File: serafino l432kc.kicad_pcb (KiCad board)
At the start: 4 copper layers, 17.8 x 35.6 mm, 34 parts, among them J1 USB_B_Micro, J2 Conn_01x14, J3 Conn_01x14, Q1 SI3401A-TP, SW1 SW_Push, SW2 SW_Push, U1 AP2112K-3.3, U2 USBLC6-2SC6, U3 STM32L432KCUx, Y1 32.768K

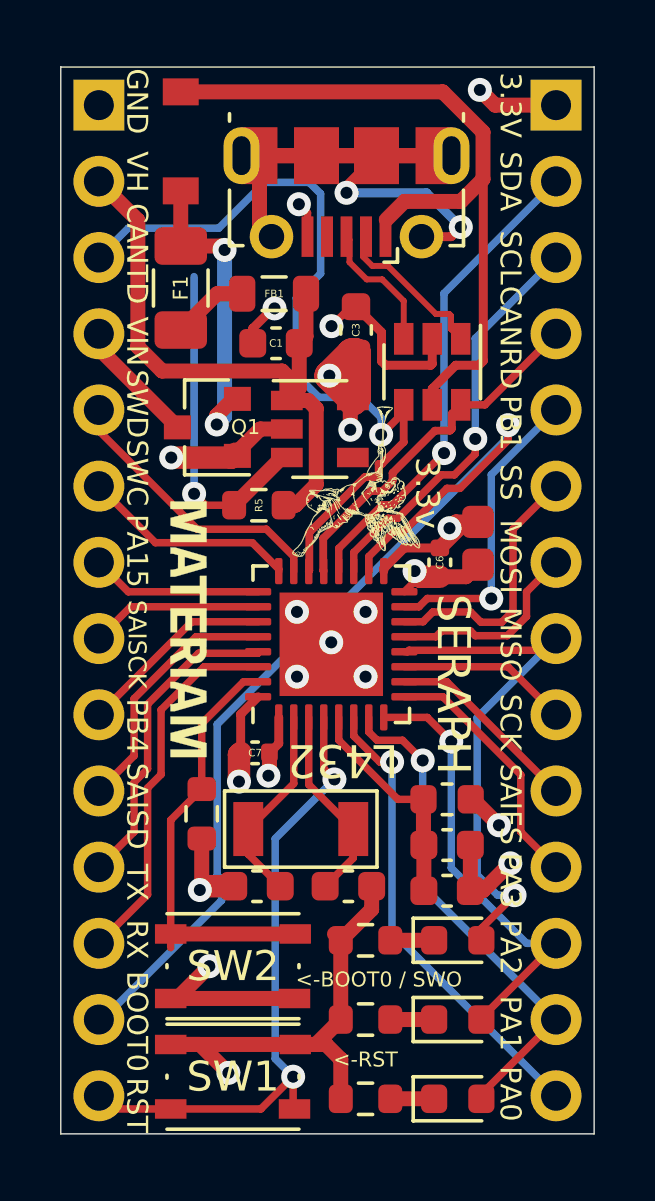
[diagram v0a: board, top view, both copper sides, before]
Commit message: Finished back labels
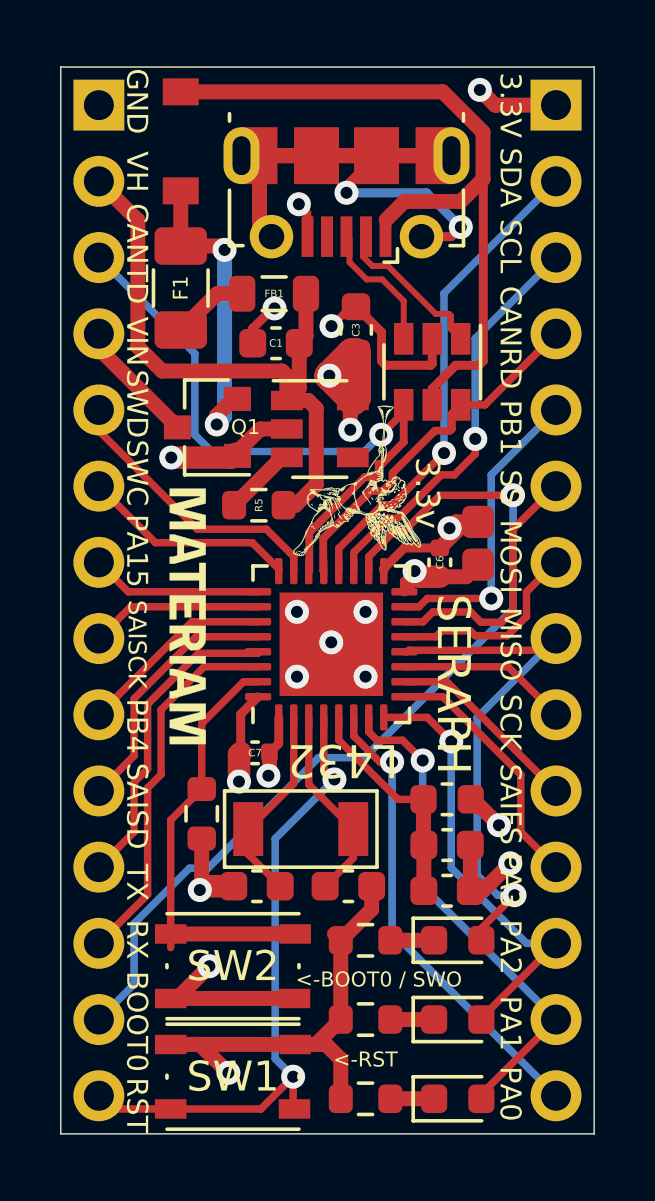
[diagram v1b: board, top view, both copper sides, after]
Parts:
- removed the G*** at (197.5, 98.0)
- moved G*** 0.43 mm to (191.7, 109.4)
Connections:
- net EN renamed Net-(R5-Pad2)
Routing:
- net Net-(R5-Pad2): track 11.1 -> 2.42 mm, vias 1 -> 0
- net CAN_TD: track 27.4 -> 22.4 mm
- net PA8: track 33.0 -> 30.6 mm
- net GND: track 42.2 -> 43.7 mm
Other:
- board text added: "* STM32L432KC ARM Cortex M4 * 64KB SRAM/256KB Flash/80Mhz * Max Supply Voltage Vin: 6.0v * Power Supply Max Iout: 600ma * Source/Sink per pin <= 20ma * Source/Sink all pins <= 100ma Press RESET while holding BOOT0 to enter DFU mode."
- board text removed: "* STM32L432KC ARM Cortex M4 * 64KB SRAM/256KB Flash/80Mhz * Max Supply Voltage Vin: 6.0v * Power Supply Max Iout: 600ma * Press RESET while holding BOOT0 to enter DFU mode."
